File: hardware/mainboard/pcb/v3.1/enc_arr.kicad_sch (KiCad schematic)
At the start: 24 parts, among them SW1 RotaryEncoder_Switch, SW2 RotaryEncoder_Switch, SW3 RotaryEncoder_Switch, SW4 RotaryEncoder_Switch

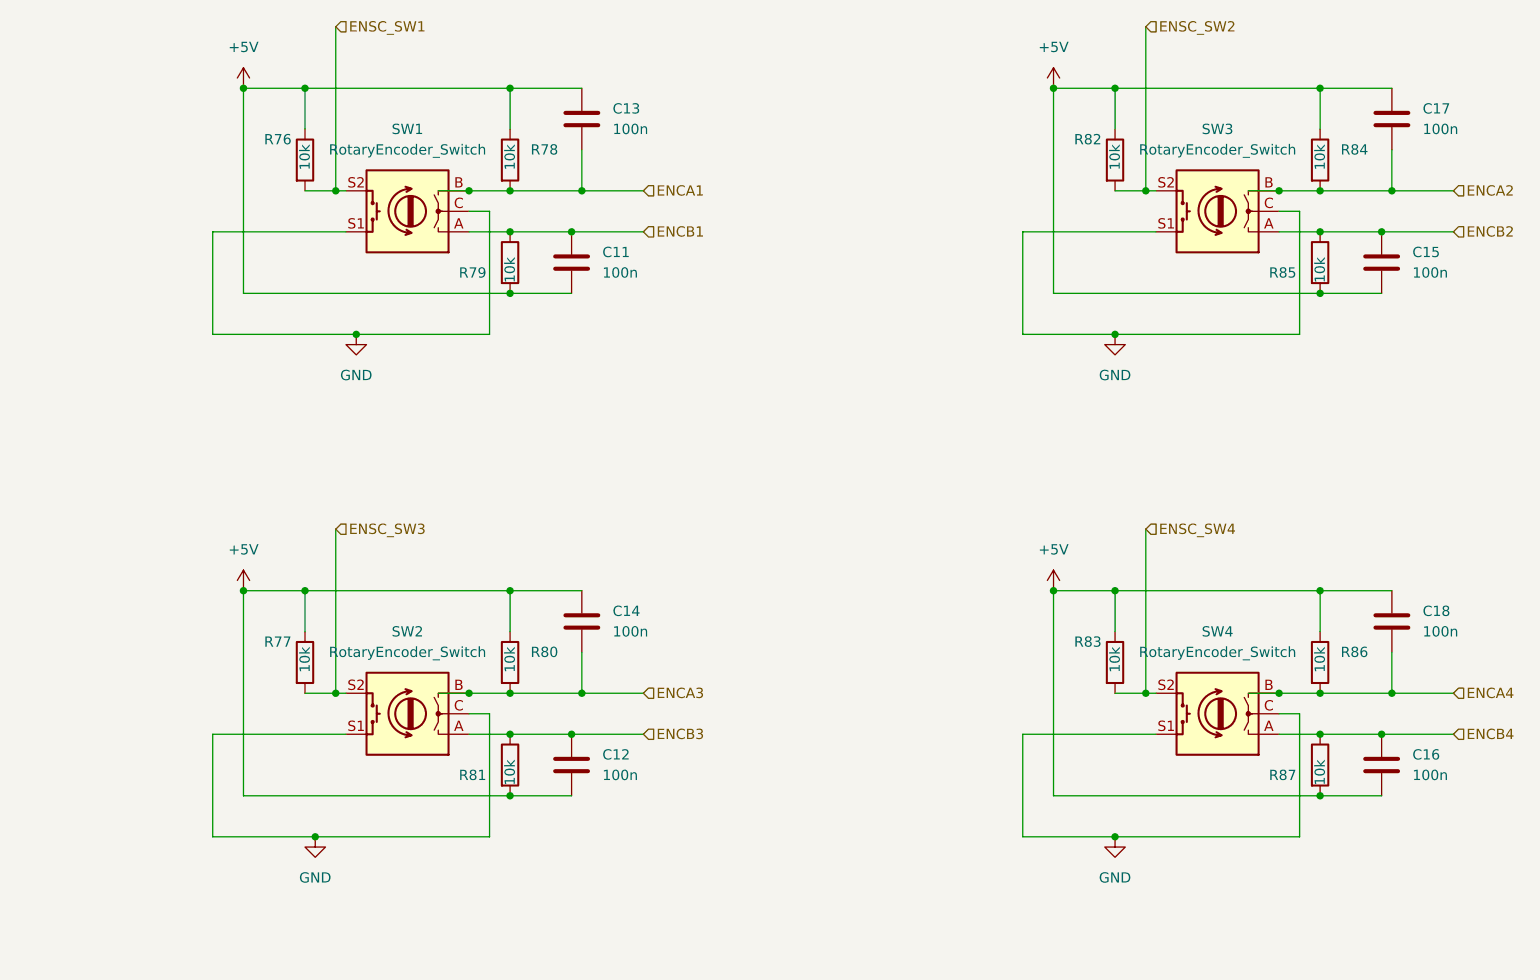
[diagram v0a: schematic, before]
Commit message: .
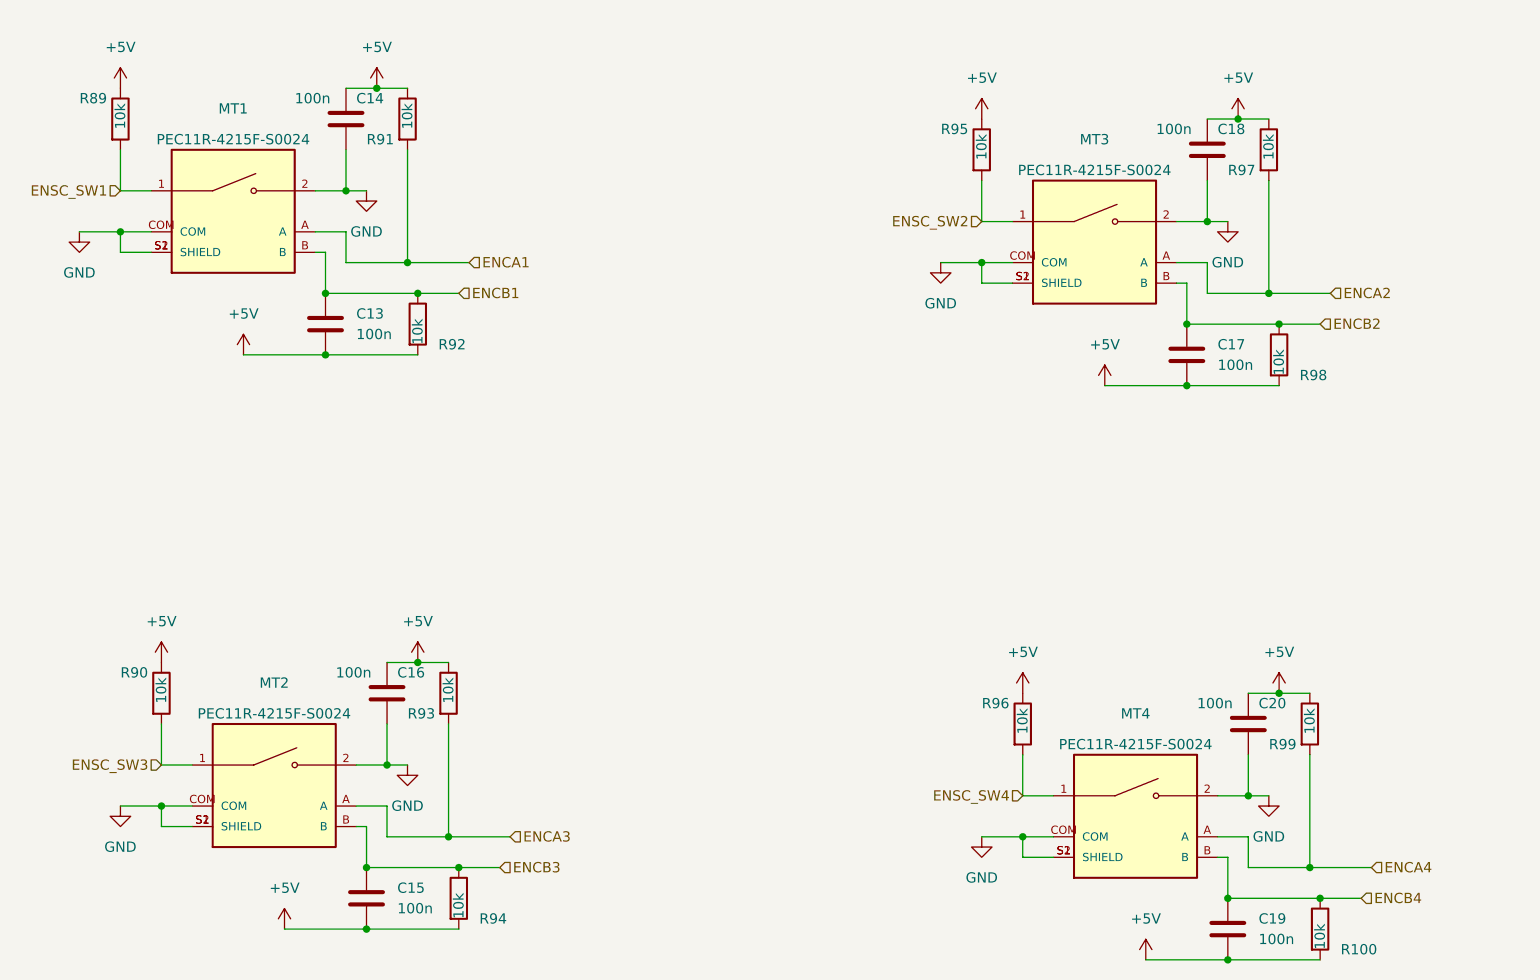
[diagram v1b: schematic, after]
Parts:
- removed C12, C14: 100n, Capacitor_SMD:C_1206_3216Metric_Pad1.33x1.80mm_HandSolder, symbol Device:C
- removed R77, R80, R81, R82, R83, R84, R85, R86, R87: 10k, Resistor_SMD:R_1206_3216Metric_Pad1.30x1.75mm_HandSolder, symbol Device:R
- removed SW1, SW2, SW3, SW4: RotaryEncoder_Switch, 3dAudioFoot:PEC11R4230KS0024, symbol Device:RotaryEncoder_Switch
- added C19, C20: 100n, Capacitor_SMD:C_1206_3216Metric_Pad1.33x1.80mm_HandSolder, symbol Device:C
- added MT1, MT2, MT3, MT4: PEC11R-4215F-S0024, 3dAudioFoot:XDCR_PEC11R-4215F-S0024, symbol 3dAudioSym:PEC11R-4215F-S0024
- added R100, R90, R93, R94, R95, R96, R97, R98, R99: 10k, Resistor_SMD:R_1206_3216Metric_Pad1.30x1.75mm_HandSolder, symbol Device:R
- renumbered C11 to C13, C13 to C14, R76 to R89, R78 to R91, R79 to R92
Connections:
- net +5V: now also C16.1, C17.2, C19.2, C20.1, R100.2, R90.1, R93.1, R94.2, R95.1, R96.1, R97.1, R98.2, R99.1; no longer C16.2, C17.1
- net ENCA1: now also MT1.A; no longer C14.2
- net ENCA2: now also MT3.A, R97.2; no longer C17.2
- net ENCA3: now also MT2.A, R93.2
- net ENCA4: now also MT4.A, R99.2; no longer C18.2
- net ENCB1: now also MT1.B
- net ENCB2: now also C17.1, MT3.B, R98.1; no longer C15.1
- net ENCB3: now also C15.1, MT2.B, R94.1
- net ENCB4: now also C19.1, MT4.B, R100.1; no longer C16.1
- net ENSC_SW1: now also MT1.1
- net ENSC_SW2: now also MT3.1, R95.2
- net ENSC_SW3: now also MT2.1, R90.2
- net ENSC_SW4: now also MT4.1, R96.2
- net GND: now also C14.2, C16.2, C18.2, C20.2, MT1.2, MT1.COM, MT1.S1 (SHIELD), MT1.S2 (SHIELD), MT2.2, MT2.COM, MT2.S1 (SHIELD), MT2.S2 (SHIELD), MT3.2, MT3.COM, MT3.S1 (SHIELD), MT3.S2 (SHIELD), MT4.2, MT4.COM, MT4.S1 (SHIELD), MT4.S2 (SHIELD)
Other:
- moved on the sheet: C13, C14, R89, R91, R92
